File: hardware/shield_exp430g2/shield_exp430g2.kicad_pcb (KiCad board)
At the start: 2 copper layers, 58.7 x 51.2 mm, 49 parts, among them J1 Digital, J14 Conn_01x04_Male, J2 Digital, J9 Conn_02x13_Odd_Even, M1 Conn_01x02_Male, M1N Conn_01x02_Male, M2 Conn_01x02_Male, M2N Conn_01x02_Male, Q1 2N7002, Q2 2N7002, U1 NCP1117-3.3_SOT223

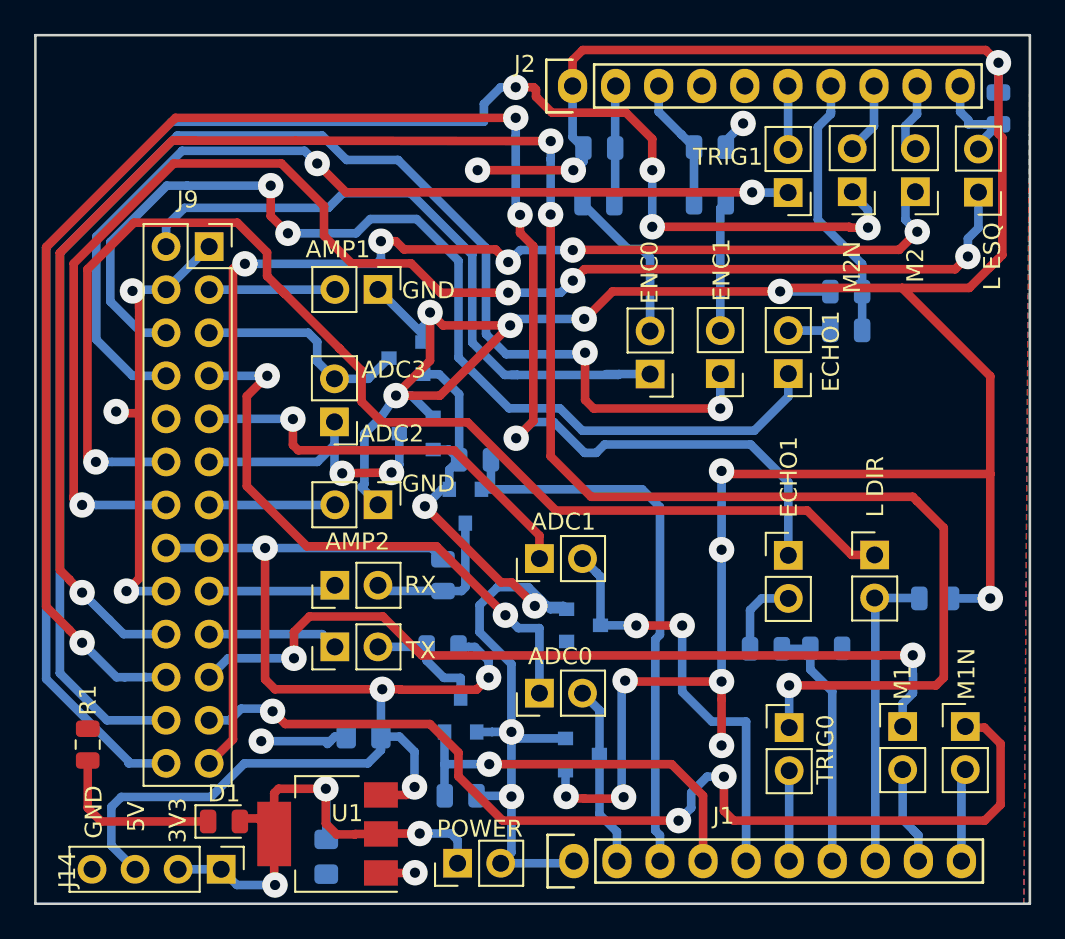
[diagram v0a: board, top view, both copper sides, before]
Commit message: Added 3d Models
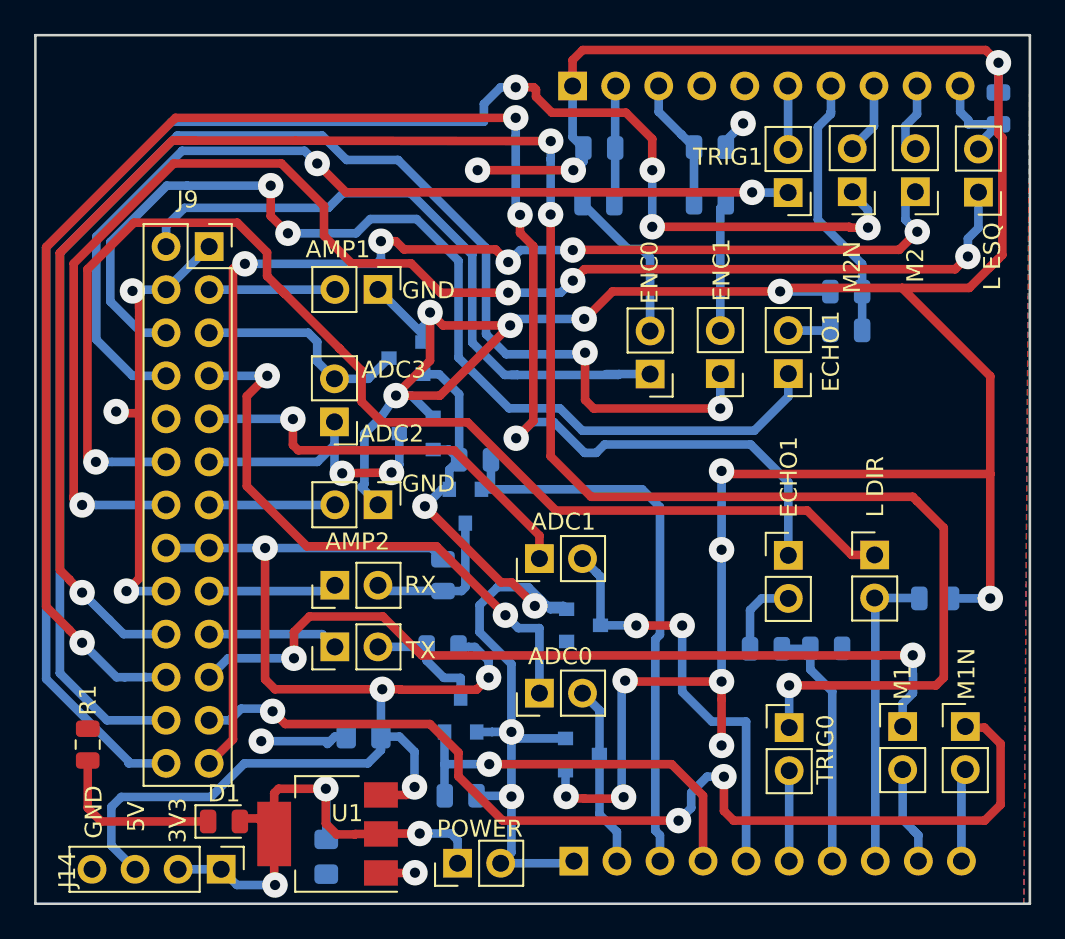
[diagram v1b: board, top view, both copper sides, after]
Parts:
- J1, J2: footprint Socket_Arduino_Uno:Socket_Strip_Arduino_1x10 -> Connector_PinHeader_2.54mm:PinHeader_1x10_P2.54mm_Vertical; moved to B.Cu
- turned J1 to 270 degrees
- turned J2 to 270 degrees
